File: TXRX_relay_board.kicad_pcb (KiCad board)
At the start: 2 copper layers, 100 x 82 mm, 80 parts, among them J1 Screw_Terminal_01x02, J2 Conn_01x08, J3 IN, J4 IN_RF_Deck, J5 OUT_RF_Deck, J6 OUT, K1 RT314A05, K2 RT314A05, Q1 BC807, Q2 BC807, Q3 BC846, Q4 BC807, Q5 BC807, Q6 BC807, U1 OP07, U2 AMS1117-5.0

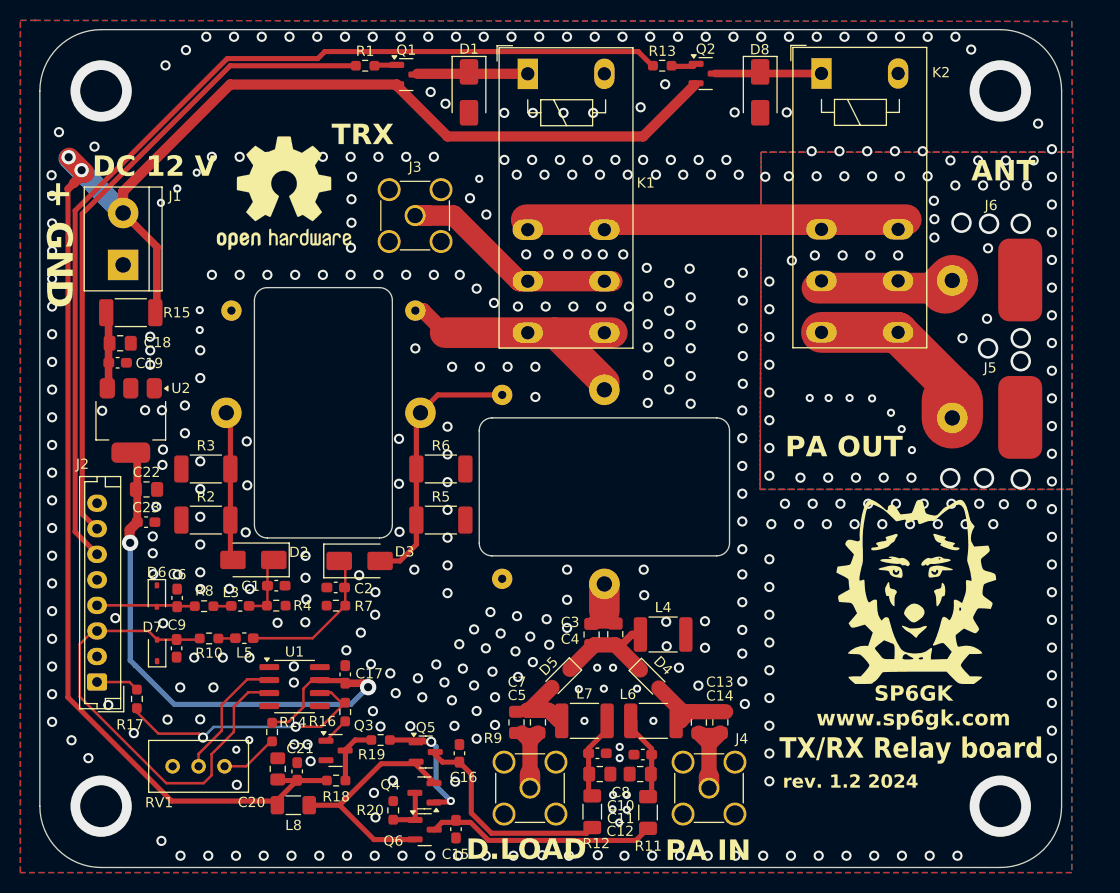
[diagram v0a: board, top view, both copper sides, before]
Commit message: Ready to Order
Minor updates in preparation to order PCBs and components
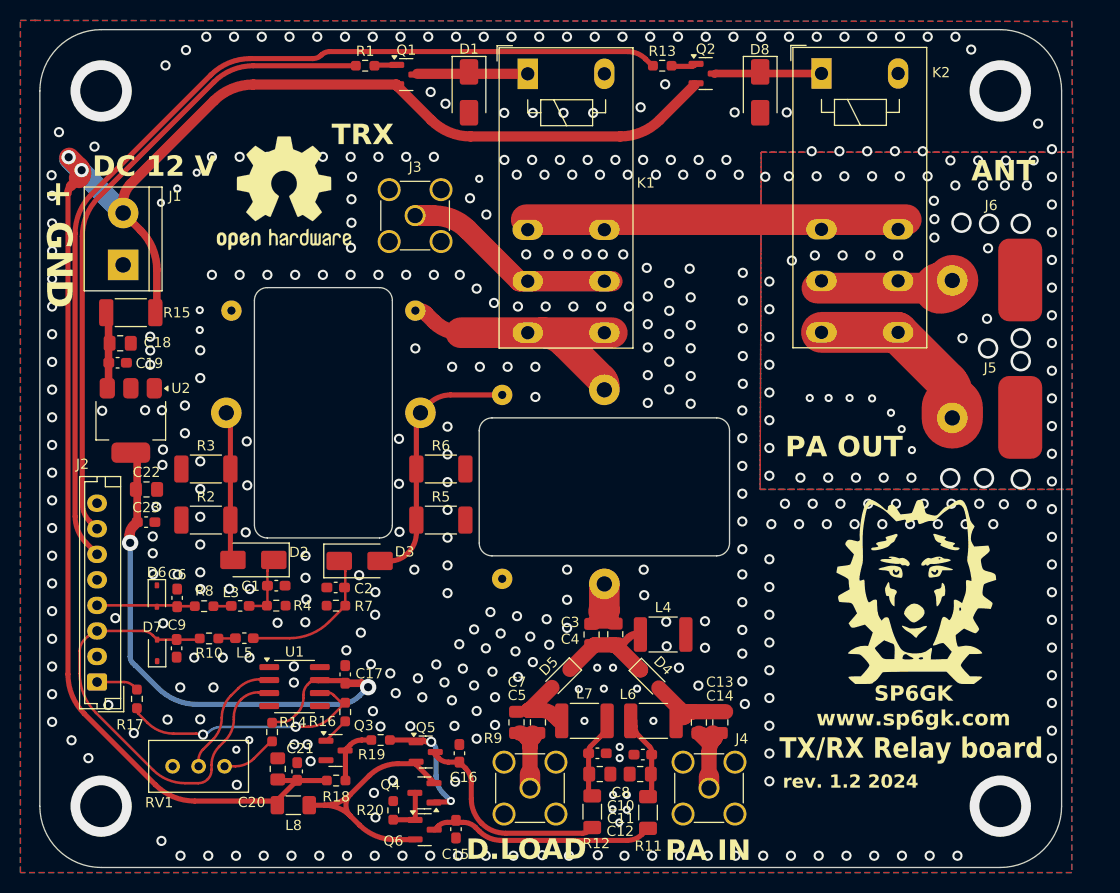
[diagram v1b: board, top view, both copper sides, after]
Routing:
- net Net-(Q4-E): track 23.5 -> 26.5 mm
- net +12V: track 171.3 -> 169.1 mm
- net FWD_PWR: track 45.9 -> 44.7 mm
- net Rel2: track 98.1 -> 97.2 mm
- net Net-(J4-In): track 10.5 -> 9.56 mm
- net +5V: track 58.5 -> 57.6 mm
- net Net-(R16-Pad2): track 25.8 -> 25.1 mm
- net Rel1: track 64.2 -> 63.6 mm
- net Bias: track 21.1 -> 20.6 mm
- net Net-(U1--): track 12.9 -> 12.4 mm
